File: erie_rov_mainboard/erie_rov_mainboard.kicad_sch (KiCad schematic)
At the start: 32 parts, among them J1 1761426-1, J10 Telem2, J11 I2C, J12 GPS, J13 SERIAL4/5, J14 RDR, J15 Expansion, J2 BATT, J3 PANEL, J4 BATT_CC, J5 LOAD, J6 855135002, J7 MR30-M, J8 ESC 12V, J9 Telem1, Q1 FDV303N, Q2 FDV303N, Q3 AO3401A, U1 Teensy4.0, U2 MAX3232CUE+T, U3 TSR 2-2450

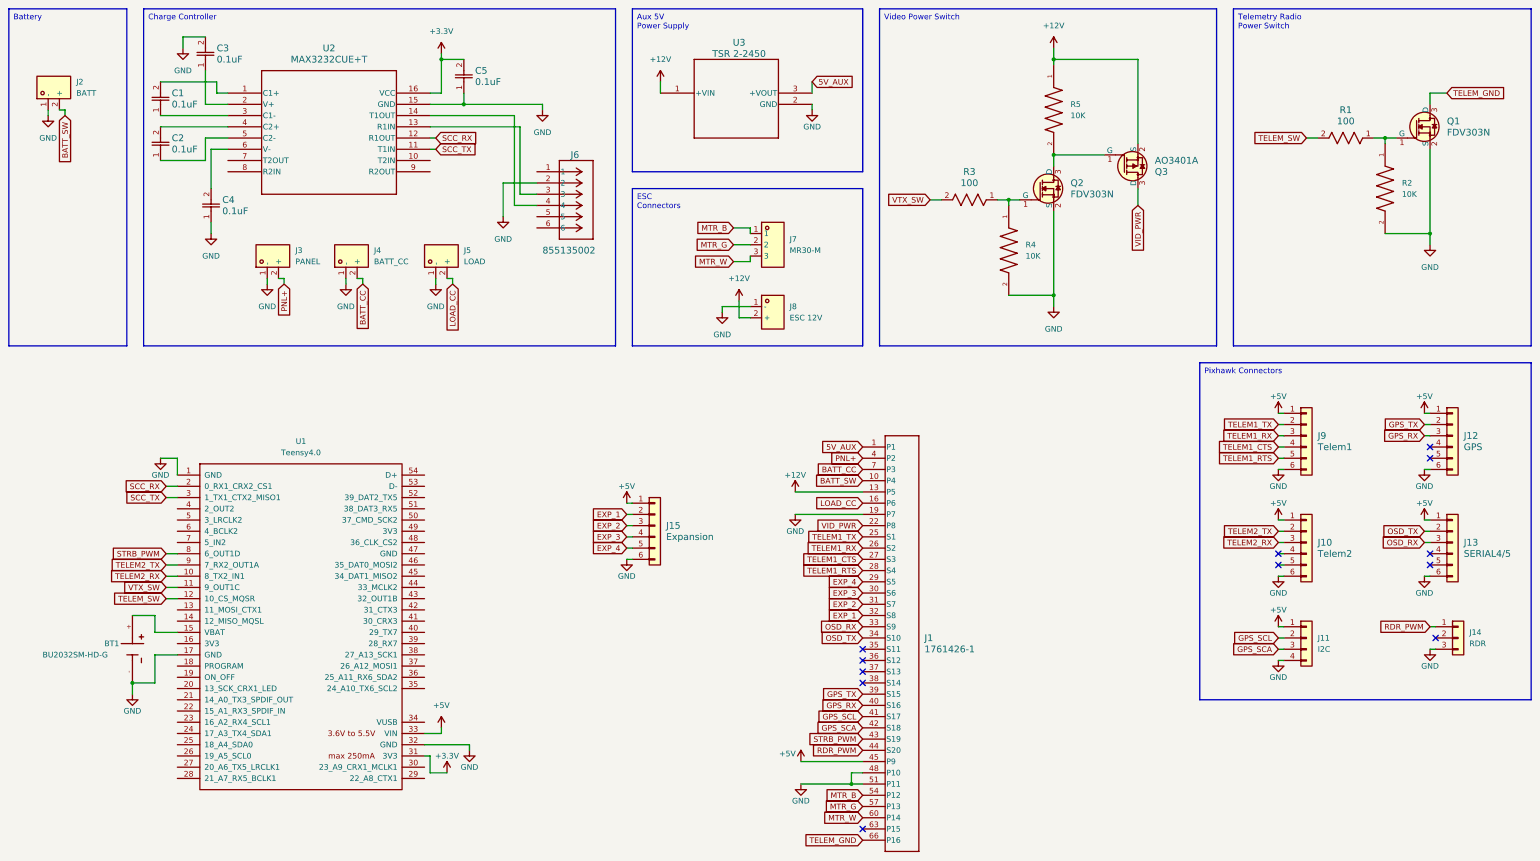
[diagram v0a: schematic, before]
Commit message: Final changes before ordering v1.0
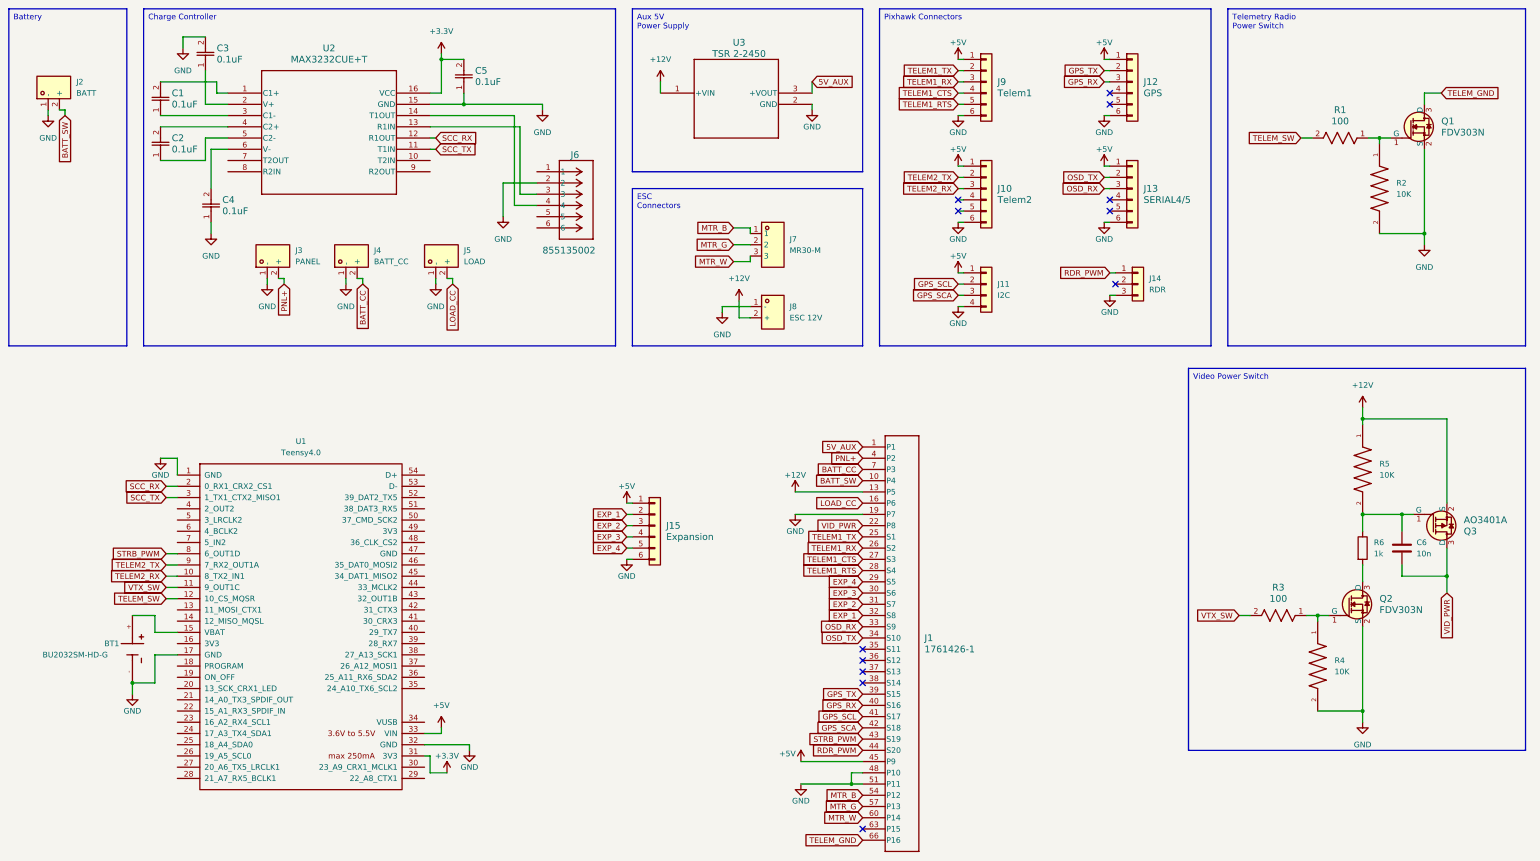
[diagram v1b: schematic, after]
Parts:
- added C6: 10n, Capacitor_SMD:C_0805_2012Metric_Pad1.18x1.45mm_HandSolder, symbol Device:C
- added R6: 1k, Resistor_SMD:R_0805_2012Metric_Pad1.20x1.40mm_HandSolder, symbol Device:R
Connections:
- net VID_PWR: now also C6.2
- net at Q3.1 (G), R5.2: now also C6.1, R6.1; no longer Q2.3 (D)
- new net: Q2.3 (D), R6.2
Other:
- moved on the sheet: J10, J11, J12, J13, J14, J9, Q1, Q2, Q3, R1, R2, R3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
